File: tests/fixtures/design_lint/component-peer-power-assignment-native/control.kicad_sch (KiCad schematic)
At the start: 2 parts, among them U1 Synthetic power module, U2 Synthetic power module

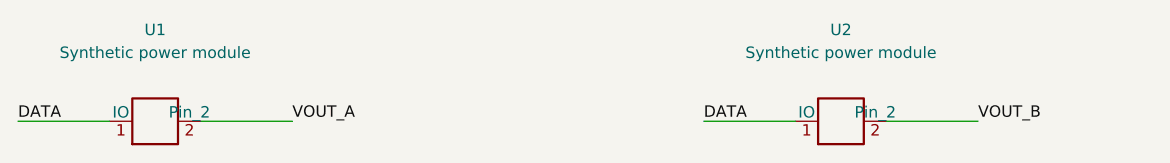
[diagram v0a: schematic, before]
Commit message: Add comparable peer pin lint gates
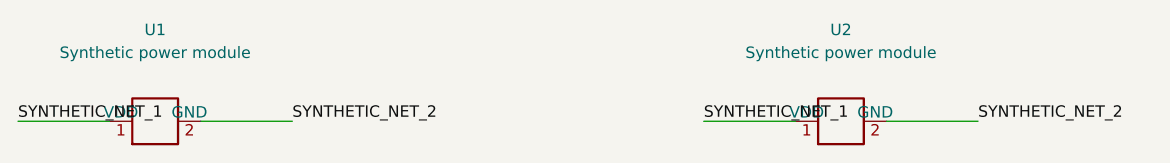
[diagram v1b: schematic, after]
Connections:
- net VOUT_B is gone; now on net SYNTHETIC_NET_2: U2.2 (GND)
- net DATA renamed SYNTHETIC_NET_1
- net VOUT_A renamed SYNTHETIC_NET_2
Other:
- title: Synthetic power-output peer control -> Synthetic power-pin assignment peer control
- moved on the sheet: U1, U2
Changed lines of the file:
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@@
 (kicad_sch (version 20231120) (generator "eeschema")
   (paper "A4")
-  (title_block (title "Synthetic power-output peer control")
+  (title_block (title "Synthetic power-pin assignment peer control")
     (comment 1 "NOT FOR MANUFACTURE - tooling fixture"))
   (symbol (lib_id "Synthetic:PowerModule") (at 88.9 78.74 0) (unit 1)
@@
     (pin "1")
     (pin "2")
-    (instances (project "Synthetic peer power-output fixture" (path "/58fe9fab-a929-4a44-a7fd-b83188082220" (reference "U1") (unit 1))))
+    (instances (project "Synthetic peer power-pin assignment fixture" (path "/58fe9fab-a929-4a44-a7fd-b83188082220" (reference "U1") (unit 1))))
   )
   (symbol (lib_id "Synthetic:PowerModuleAlias") (at 165.1 78.74 0) (unit 1)
@@
     (pin "1")
     (pin "2")
-    (instances (project "Synthetic peer power-output fixture" (path "/58fe9fab-a929-4a44-a7fd-b83188082220" (reference "U2") (unit 1))))
+    (instances (project "Synthetic peer power-pin assignment fixture" (path "/58fe9fab-a929-4a44-a7fd-b83188082220" (reference "U2") (unit 1))))
   )
   (wire (pts (xy 83.82 78.74) (xy 73.66 78.74))
     (stroke (width 0) (type default))
 )
-  (label "DATA" (at 73.66 78.74 0)
+  (label "SYNTHETIC_NET_1" (at 73.66 78.74 0)
     (effects (font (size 1.27 1.27)) (justify left bottom))
 )
@@
     (stroke (width 0) (type default))
 )
-  (label "DATA" (at 149.86 78.74 0)
+  (label "SYNTHETIC_NET_1" (at 149.86 78.74 0)
     (effects (font (size 1.27 1.27)) (justify left bottom))
 )
@@
     (stroke (width 0) (type default))
 )
-  (label "VOUT_A" (at 104.14 78.74 0)
+  (label "SYNTHETIC_NET_2" (at 104.14 78.74 0)
     (effects (font (size 1.27 1.27)) (justify left bottom))
 )
@@
     (stroke (width 0) (type default))
 )
-  (label "VOUT_B" (at 180.34 78.74 0)
+  (label "SYNTHETIC_NET_2" (at 180.34 78.74 0)
     (effects (font (size 1.27 1.27)) (justify left bottom))
 )
